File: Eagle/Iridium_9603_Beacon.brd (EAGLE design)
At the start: 50.8 x 71.1 mm, 64 parts, among them J1 SS4-10-3.50-X-D, Q1 DMG3415U-7, U1 MCP111T-195I/TT, U2 SPX3819-3.3, U3 LTC3225EDDB#TRMPBF, U4 MPL3115A2LGA8, U5 ATSAMD21G18_QFN, U6 SAM-M8Q, X1 32.768

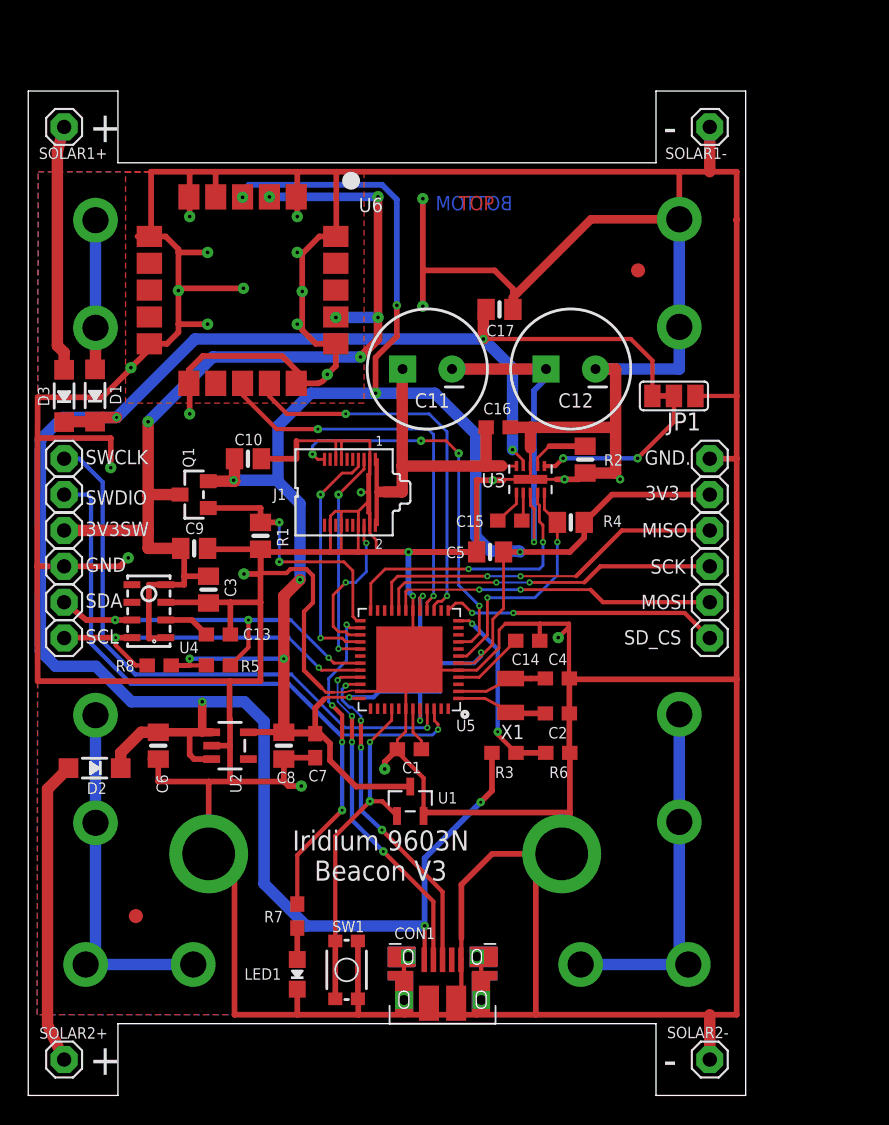
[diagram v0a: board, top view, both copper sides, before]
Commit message: Initial update for V4 - still work in progress
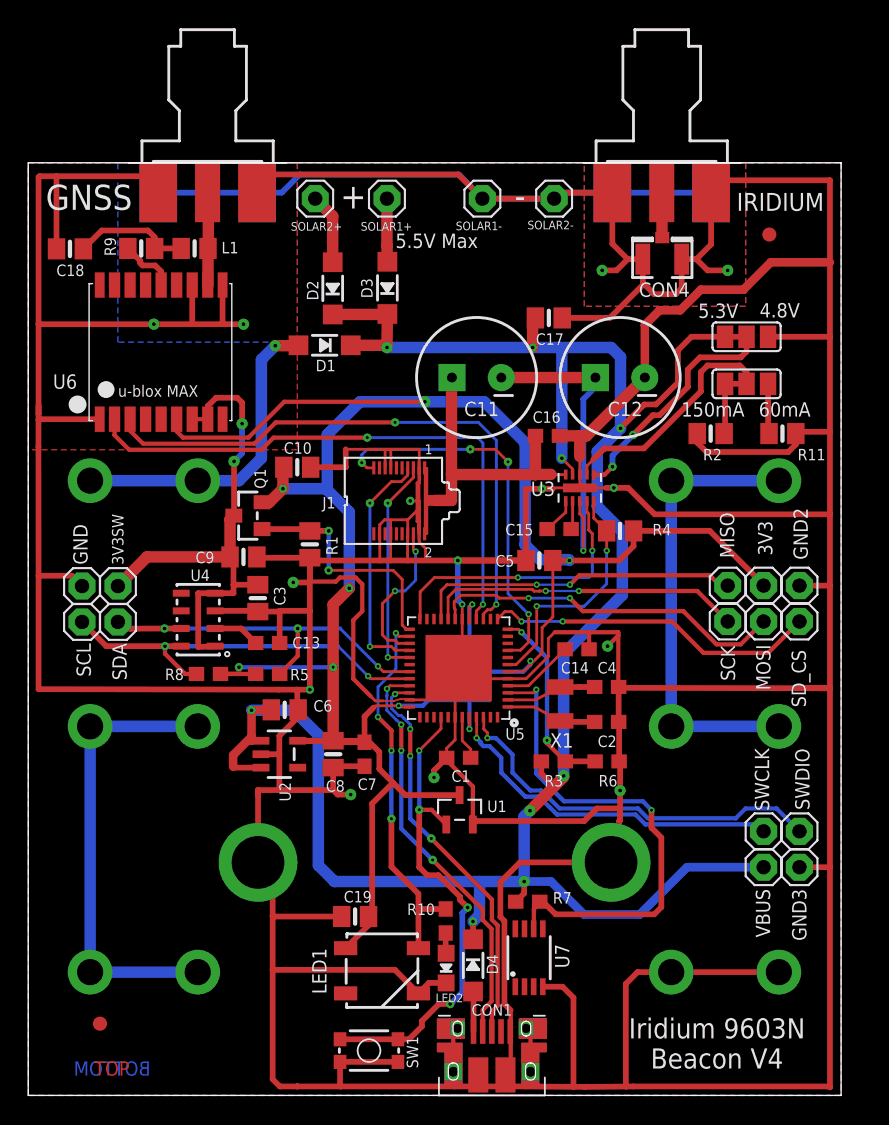
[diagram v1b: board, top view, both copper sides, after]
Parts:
- removed GND.: (no value), adafruit:1X01
- added C18: 10nF, microbuilder:0805-NO
- added C19: 10uF, microbuilder:0805-NO
- added CON4: uFL, microbuilder:U.FL
- added D4: MBR120, microbuilder:SOD-123
- added GND2, GND3, VBUS: (no value), adafruit:1X01
- added GNSS, IRIDIUM: SMA-142-0711-821/826, con-coax:J502-ND-142-0711-821/826
- added JP2: (no value), SparkFun-Passives:PAD-JUMPER-3-2OF3_NC_BY_TRACE_YES_SILK_LARGE
- added L1: 33nH, microbuilder:0805-NO
- added LED2: RED, microbuilder:CHIPLED_0805_NOOUTLINE
- added R10: 2.2K, microbuilder:0603-NO
- added R11: 30K, microbuilder:0805-NO
- added R9: 10 ohm, microbuilder:0805-NO
- added U7: LT1634-1,25BMCMS8, linear-technology:MSOP8
- BAT1, BAT2, BAT3: device SparkFun-Electromechanical:BATTERY-AAA-KEYSTONE82 -> SparkFun-Electromechanical:BATTERY-AAA-KEYSTONE92
- LED1: value RED -> (none); device microbuilder:CHIPLED_0805_NOOUTLINE -> SparkFun-LED:WS2812B
- R2: value 30K -> 12K
- R7: value 2.2K -> 47k
- U1: value MCP111T-195I/TT -> MCP111T-240E/TT
- U6: value SAM-M8Q -> MAX-M8; device ubloxLib:SAM-M8Q -> ubloxLib:MAX-M8
- moved SOLAR2+ 63.5 mm to (20.3, 63.5)
- moved SOLAR2- 61.9 mm to (37.2, 63.5)
- moved SWDIO 57.3 mm to (54.6, 18.7), turned to 90 degrees
- moved SWCLK 56.1 mm to (52.1, 18.7), turned to 90 degrees
- moved D2 37.9 mm to (21.6, 57.1), turned to 90 degrees
- moved BAT3 36.4 mm to (28.8, 8.73), turned to 180 degrees
- moved BAT1 24.2 mm to (28.8, 43.5), turned to 180 degrees
- moved D3 24.1 mm to (25.4, 57.2)
- moved SOLAR1+ 23.4 mm to (25.4, 63.5)
- moved BAT2 17.2 mm to (28.8, 26.1), turned to 0 degrees
- moved SOLAR1- 16.9 mm to (32.2, 63.5)
- moved D1 16.6 mm to (21.0, 53.1), turned to 180 degrees
- moved R7 16.4 mm to (35.4, 13.7), turned to 0 degrees
- moved FD2 9.64 mm to (52.5, 61.0)
- moved C6 9.31 mm to (18.2, 27.3), turned to 0 degrees
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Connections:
- new net 9_V_RESET_N: U6.9_RESET_N
- new net GPS_ANT: GNSS.1, L1.2, U6.11_RF_IN
- new net N$1: C18.1, L1.1, R9.1
- new net N$16: CON1.VBUS, D4.A
- new net N$17: JP2.3, R2.2
- new net N$18: JP2.1, R11.2
- new net N$3: LED2.A, R10.2
- new net VCC_RF: R9.2, U6.14_VCC_RF
- net +3V3: now also C19.1, LED1.1, U6.6_V_BCKP; no longer U6.3
- net 3V3SW: now also U6.7_VCC_IO, U6.8_VCC; no longer U6.17, U6.2
- net A0: now also R7.2, U7.6
- net D0: now also U6.2_TXD; no longer U6.13
- net D1: now also U6.3_RXD; no longer U6.14
- net D13: now also LED1.4, R10.1; no longer R7.1
- net GND: now also C18.2, C19.2, CON4.1, CON4.2, GND2.1, GND3.1, GNSS.G@1, GNSS.G@2, GNSS.G@3, GNSS.G@4, IRIDIUM.G@1, IRIDIUM.G@2, IRIDIUM.G@3, IRIDIUM.G@4, LED1.3, LED2.C, R11.1, U6.10_GND, U6.12_GND, U6.1_GND, U7.4; no longer GND..1, LED1.C, U6.1, U6.10, U6.11, U6.15, U6.16, U6.20, U6.4, U6.5, U6.6
- net N$11: now also JP2.2; no longer R2.2
- net N$2: now also CON4.3, IRIDIUM.1; no longer LED1.A, R7.2
- net VBUS: now also D4.C, R7.1, VBUS.1; no longer CON1.VBUS
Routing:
- net GND: track 633.8 -> 700.3 mm, vias 26 -> 15
- net A0: track 0.00 -> 35.7 mm, vias 0 -> 2
- net 3V3SW: track 71.1 -> 37.0 mm, vias 6 -> 2
- net N$14: track 21.5 -> 5.01 mm
- net SWCLK: track 41.6 -> 25.2 mm
- net D1: track 27.7 -> 41.5 mm
- net SWDIO: track 41.3 -> 27.7 mm
- net N$4: track 17.5 -> 4.47 mm
- net D0: track 28.2 -> 40.8 mm
- net N$11: track 4.29 -> 16.7 mm
- net VBAT: track 10.6 -> 22.8 mm, vias 0 -> 1
- net !RESET: track 24.5 -> 34.8 mm, vias 2 -> 4
- net N$1: track 0.00 -> 8.46 mm
- net +3V3: track 176.8 -> 184.2 mm, vias 12 -> 10
- net N$8: track 25.3 -> 32.6 mm
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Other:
- board size 50.8 x 71.1 mm -> 57.6 x 66 mm
- board text added: "150mA"
- board text added: "4.8V"
- board text added: "5.3V"
- board text added: "5.5V Max"
- board text added: "60mA"
- board text added: "Iridium 9603N Beacon V4"
- board text added: "Please return to:"
- board text removed: "Iridium 9603N Beacon V3"
- board text removed: "Please return to: Durham University ph-cfai-bit@durham.ac.uk"
